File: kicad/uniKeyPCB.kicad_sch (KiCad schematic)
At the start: 14 parts, among them J1 Conn_01x03_Socket, J2 Conn_01x03_Socket, J3 Conn_01x03_Socket, J4 Conn_01x03_Socket, J5 Conn_01x02_Socket, J6 Conn_01x02_Socket, J7 Conn_01x02_Socket, J8 Conn_01x02_Socket, SW1 SW_CHOC_HS, SW2 SW_MX_HS

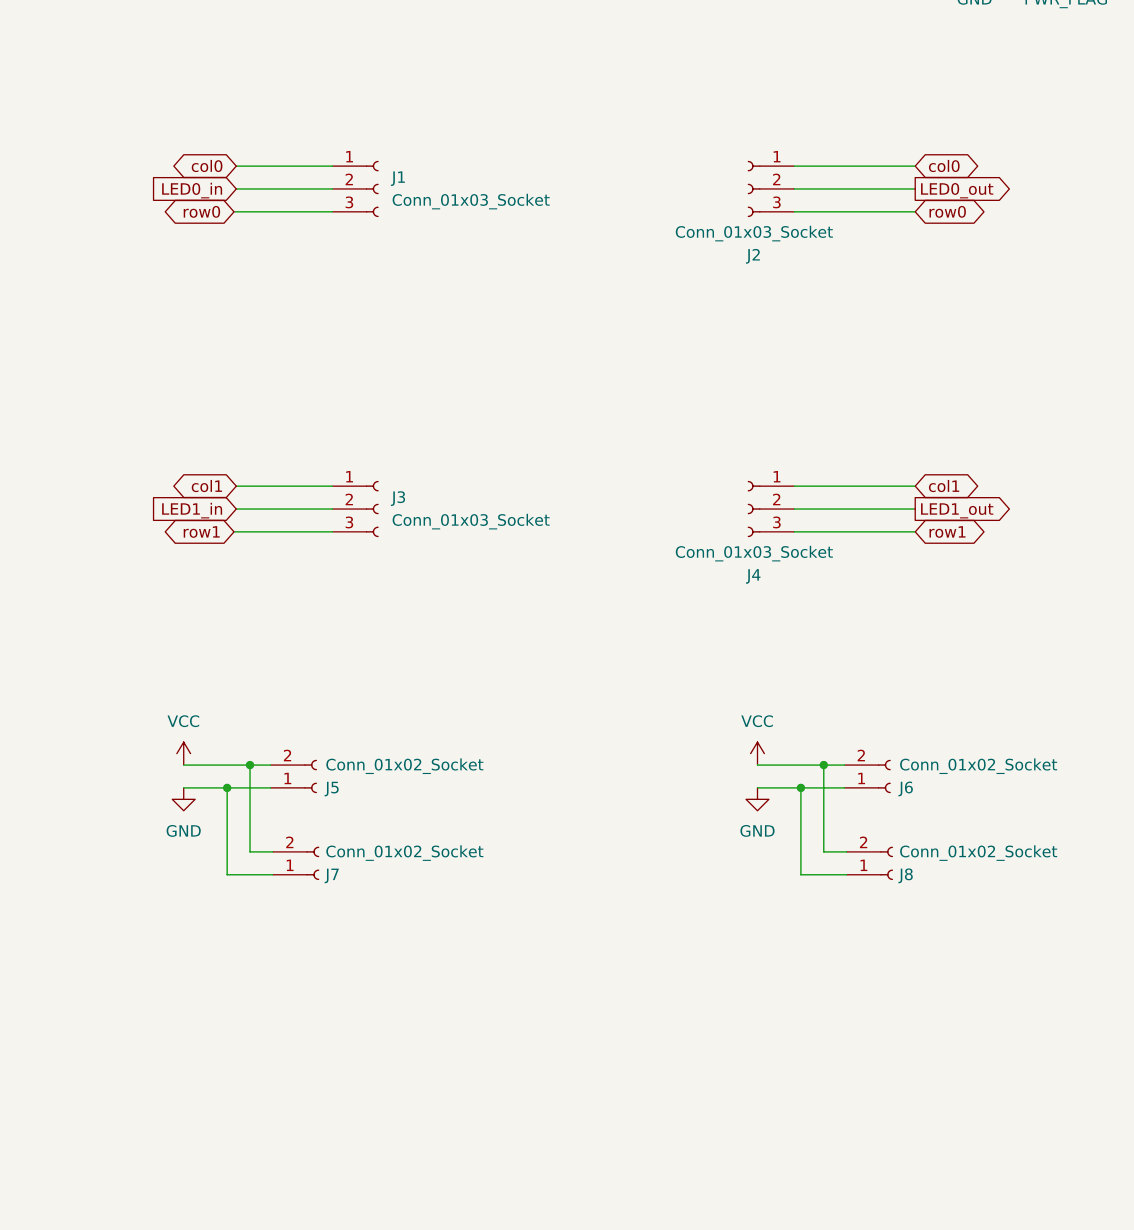
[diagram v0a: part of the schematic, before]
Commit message: more connectors
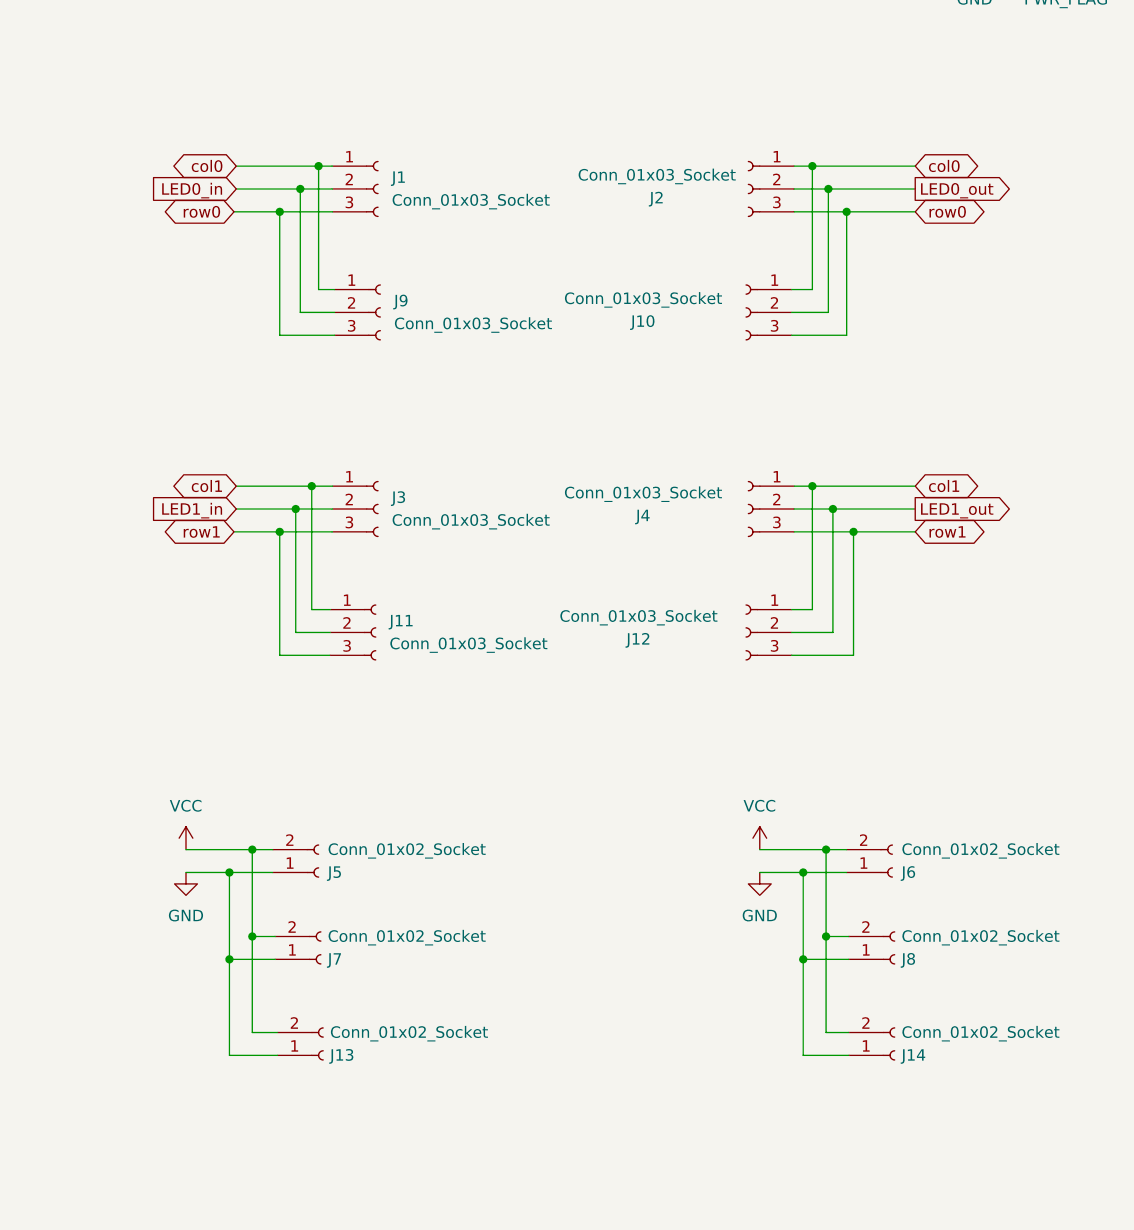
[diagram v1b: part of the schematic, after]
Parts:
- added J10, J11, J12, J9: Conn_01x03_Socket, Connector_PinHeader_2.00mm:PinHeader_1x03_P2.00mm_Vertical, symbol Connector:Conn_01x03_Socket
- added J13, J14: Conn_01x02_Socket, Connector_PinSocket_2.00mm:PinSocket_1x02_P2.00mm_Vertical, symbol Connector:Conn_01x02_Socket
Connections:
- net GND: now also J13.1 (Pin_1), J14.1 (Pin_1)
- net LED0_in: now also J9.2 (Pin_2)
- net LED0_out: now also J10.2 (Pin_2)
- net LED1_in: now also J11.2 (Pin_2)
- net LED1_out: now also J12.2 (Pin_2)
- net VCC: now also J13.2 (Pin_2), J14.2 (Pin_2)
- net col0: now also J10.1 (Pin_1), J9.1 (Pin_1)
- net col1: now also J11.1 (Pin_1), J12.1 (Pin_1)
- net row0: now also J10.3 (Pin_3), J9.3 (Pin_3)
- net row1: now also J11.3 (Pin_3), J12.3 (Pin_3)
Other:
- moved on the sheet: J5, J6, J7, J8

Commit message: Revert "more connectors (#4)"
This reverts commit e986b9c313ce46b497b00528d1270ea63e1c5e11.
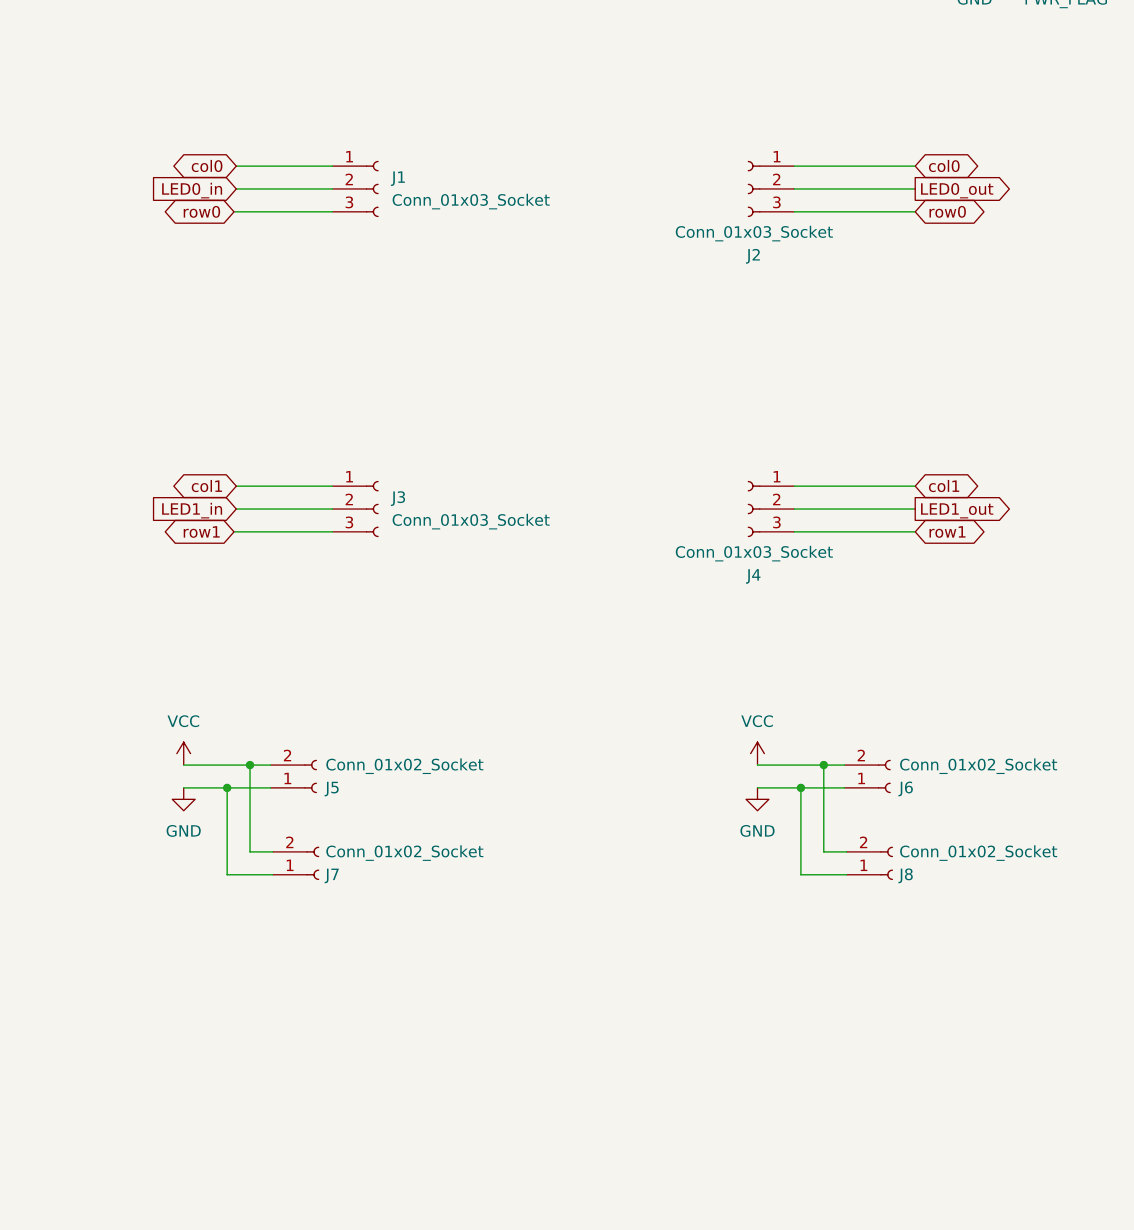
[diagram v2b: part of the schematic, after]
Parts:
- removed J10, J11, J12, J9: Conn_01x03_Socket, Connector_PinHeader_2.00mm:PinHeader_1x03_P2.00mm_Vertical, symbol Connector:Conn_01x03_Socket
- removed J13, J14: Conn_01x02_Socket, Connector_PinSocket_2.00mm:PinSocket_1x02_P2.00mm_Vertical, symbol Connector:Conn_01x02_Socket
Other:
- moved on the sheet: J5, J6, J7, J8
